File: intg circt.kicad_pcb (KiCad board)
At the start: 2 copper layers, 16.8 x 23.9 mm, 33 parts, among them J2 USB_C_Receptacle_USB2.0_16P, U1 ESP32-S3-MINI-1U, U2 MAXM86161EFD_T, U3 BMI270, U4 BQ24074RGT, U6 USBLC6-2P6, U7 MAX17048X+T10, U8 TLV75533PDBV

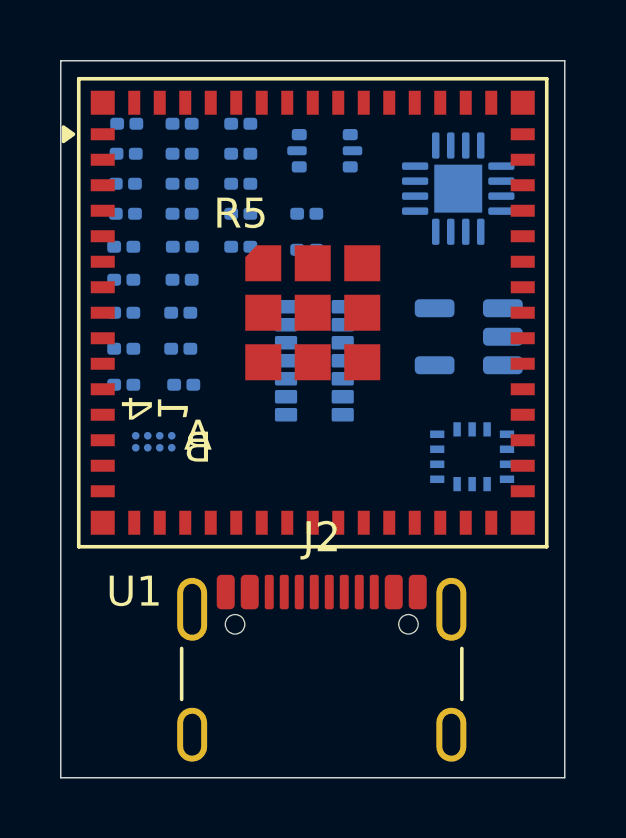
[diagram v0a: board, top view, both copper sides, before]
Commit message: change
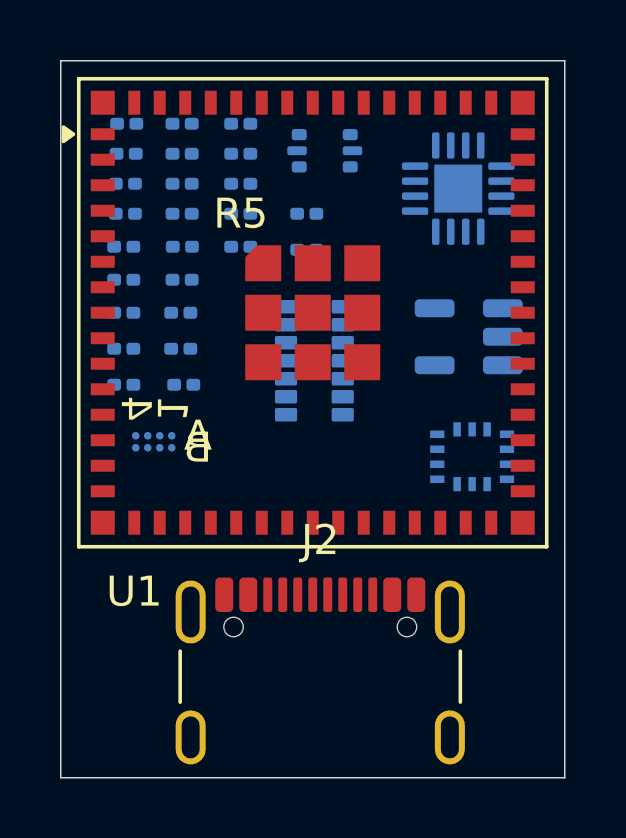
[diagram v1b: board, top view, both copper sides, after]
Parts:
- moved J2 0.10 mm to (76.8, 62.7)
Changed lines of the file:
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@@
 	(footprint "Connector_USB:USB_C_Receptacle_GCT_USB4105-xx-A_16P_TopMnt_Horizontal"
 		(layer "F.Cu")
-		(at 76.8 62.59)
+		(at 76.75 62.68)
 		(descr "USB 2.0 Type C Receptacle, GCT, 16P, top mounted, horizontal, 5A: https://gct.co/files/drawings/usb4105.pdf")
 		(tags "USB C Type-C Receptacle SMD USB 2.0 16P 16C USB4105-15-A USB4105-15-A-060 USB4105-15-A-120 USB4105-GF-A USB4105-GF-A-060 USB4105-GF-A-120")

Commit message: just tested if it works, it does i think
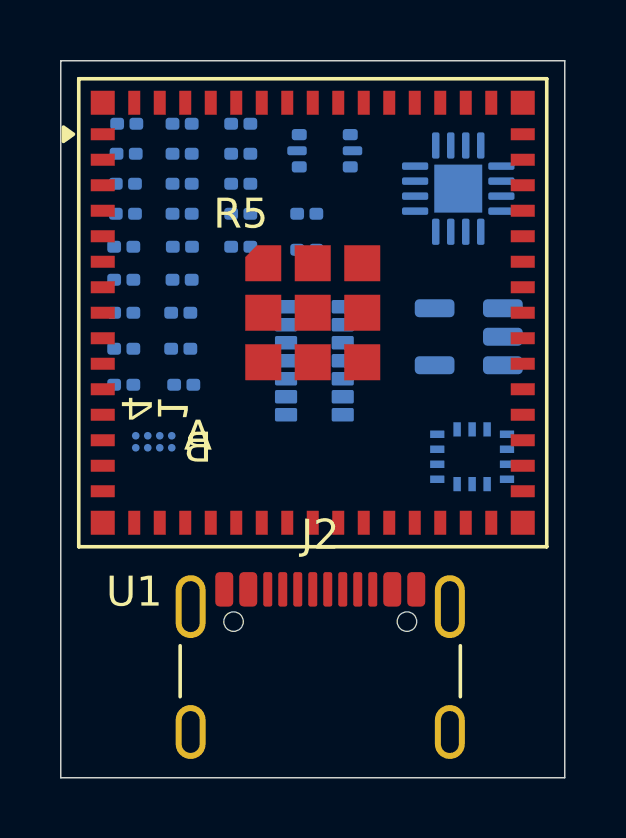
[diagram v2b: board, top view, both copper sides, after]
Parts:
- moved J2 0.18 mm to (76.8, 62.5)
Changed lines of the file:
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@@
 	(footprint "Connector_USB:USB_C_Receptacle_GCT_USB4105-xx-A_16P_TopMnt_Horizontal"
 		(layer "F.Cu")
-		(at 76.75 62.68)
+		(at 76.75 62.5)
 		(descr "USB 2.0 Type C Receptacle, GCT, 16P, top mounted, horizontal, 5A: https://gct.co/files/drawings/usb4105.pdf")
 		(tags "USB C Type-C Receptacle SMD USB 2.0 16P 16C USB4105-15-A USB4105-15-A-060 USB4105-15-A-120 USB4105-GF-A USB4105-GF-A-060 USB4105-GF-A-120")
